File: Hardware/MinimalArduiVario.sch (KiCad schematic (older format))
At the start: 35 parts, among them IC1 ATMEGA328P-A, SW1 Select, SW2 Up, SW3 Down

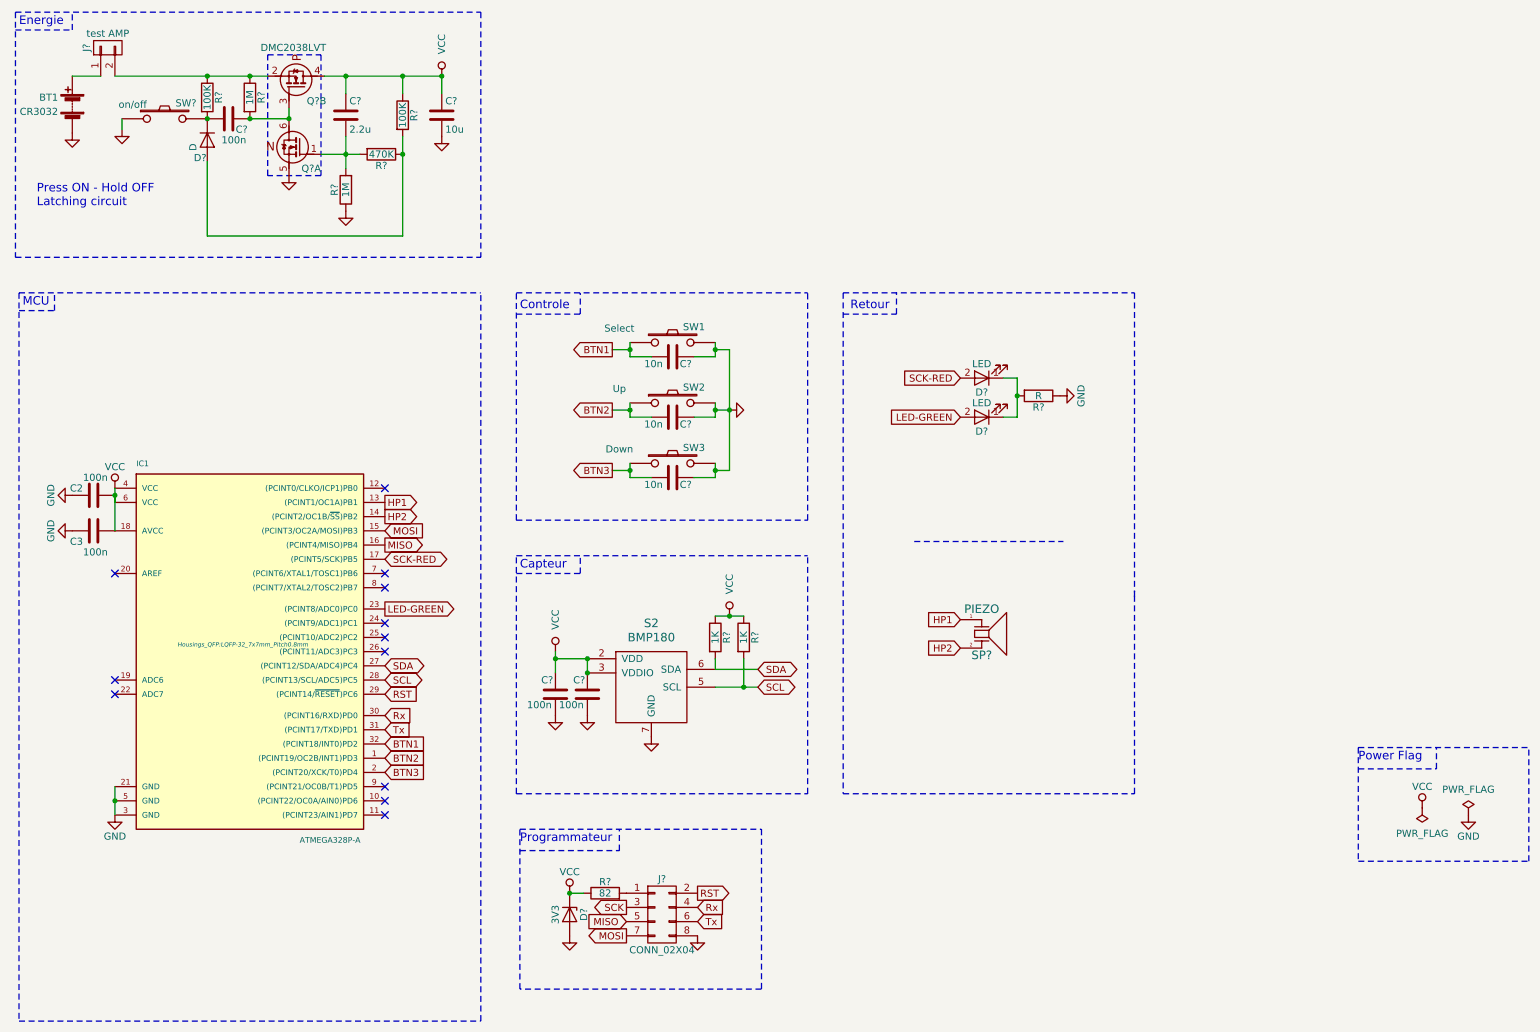
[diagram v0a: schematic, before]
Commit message: dev proto hardware v1
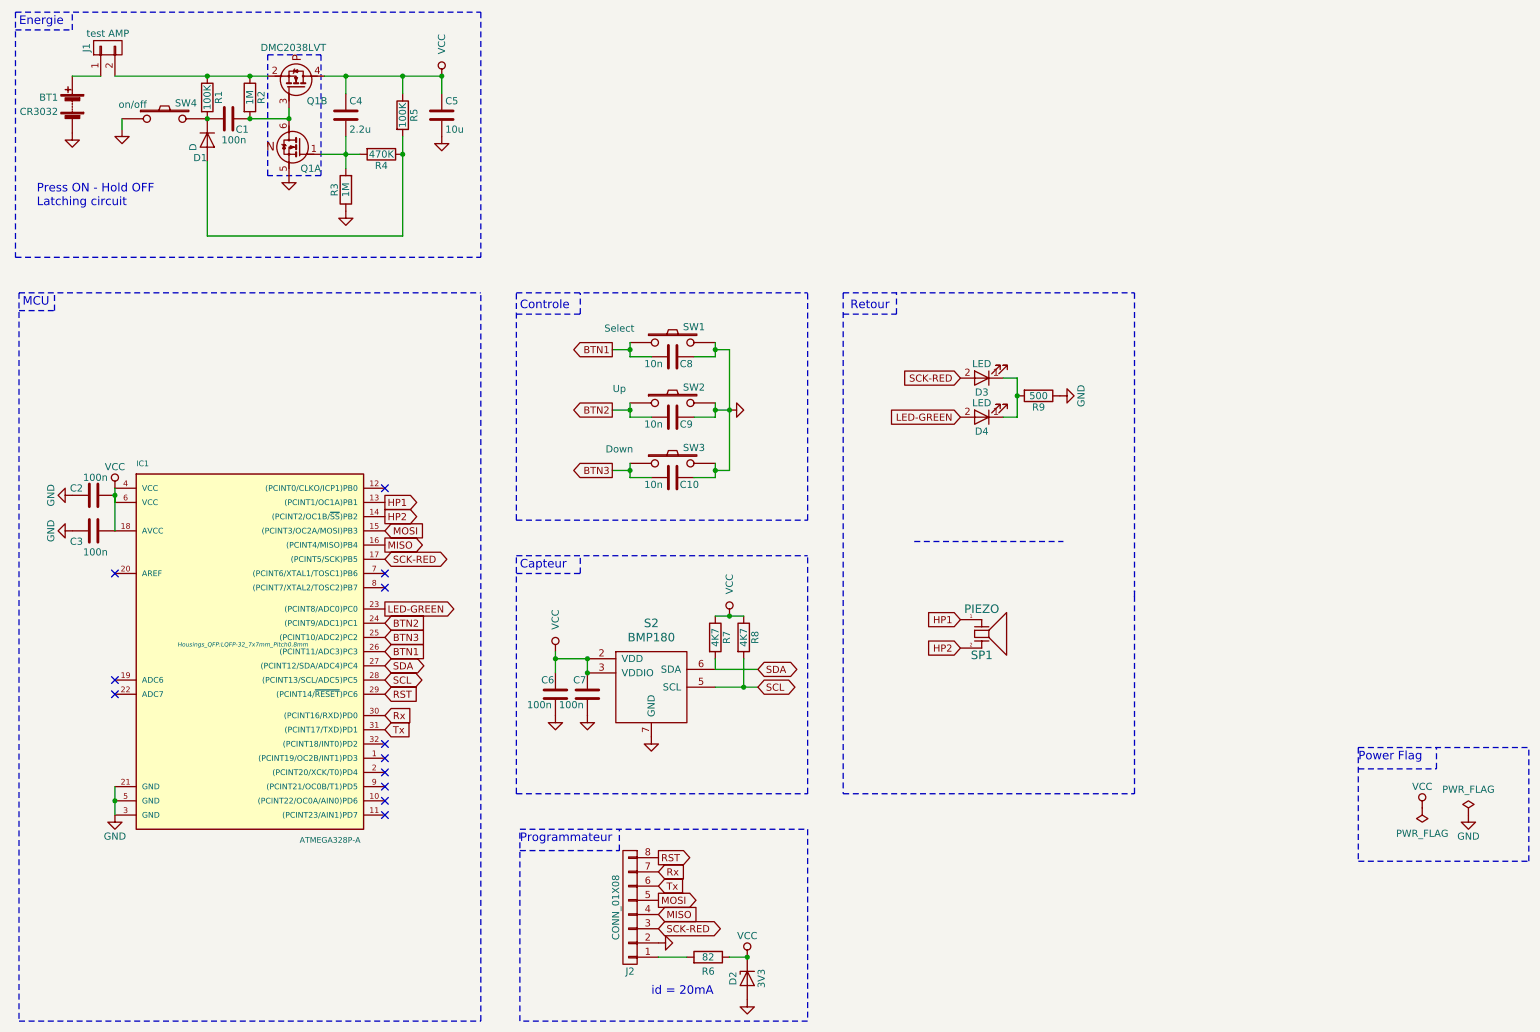
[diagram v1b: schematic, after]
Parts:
- removed J?: CONN_02X04, symbol CONN_02X04
- added J2: CONN_01X08, Pin_Headers:Pin_Header_Angled_1x08_Pitch2.54mm, symbol CONN_01X08
- R7, R8: renamed from R?; value 1K -> 4K7
- R9: renamed from R?; value R -> 500
- SW1, SW2, SW3: footprint Buttons_Switches_ThroughHole:SW_Tactile_SPST_Angled -> Buttons_Switches_THT:SW_Tactile_SPST_Angled
- SW4: renamed from SW?; footprint Buttons_Switches_ThroughHole:SW_Tactile_SPST_Angled -> Buttons_Switches_THT:SW_Tactile_SPST_Angled
- gave numbers to parts that had none: 21
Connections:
- net BTN1: now also IC1.26 ((PCINT11/ADC3)PC3); no longer IC1.32 ((PCINT18/INT0)PD2)
- net BTN2: now also IC1.24 ((PCINT9/ADC1)PC1); no longer IC1.1 ((PCINT19/OC2B/INT1)PD3)
- net BTN3: now also IC1.25 ((PCINT10/ADC2)PC2); no longer IC1.2 ((PCINT20/XCK/T0)PD4)
- net GND: now also J2.2 (P2)
- net MISO: now also J2.4 (P4)
- net MOSI: now also J2.5 (P5)
- net RST: now also J2.8 (P8)
- net Rx: now also J2.7 (P7)
- net SCK-RED: now also J2.3 (P3)
- net Tx: now also J2.6 (P6)
- net at R6.2: now also J2.1 (P1)
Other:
- note added: "id = 20mA"
- moved on the sheet: D2, R6
